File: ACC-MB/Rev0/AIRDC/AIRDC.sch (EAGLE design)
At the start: 4 parts

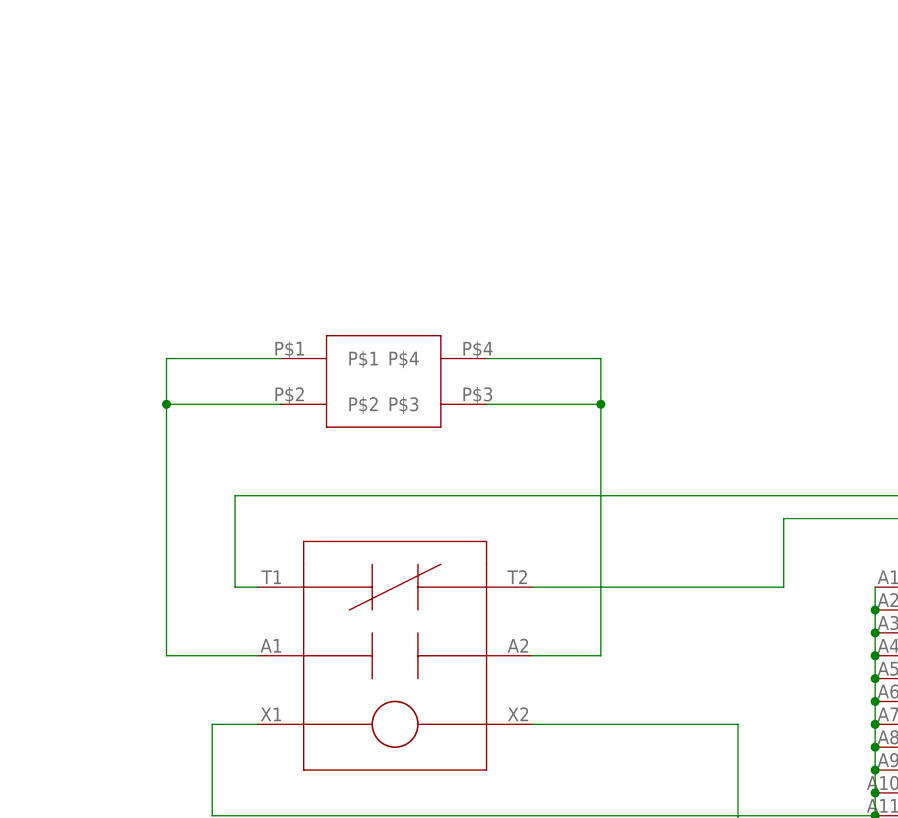
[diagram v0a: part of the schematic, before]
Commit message: update
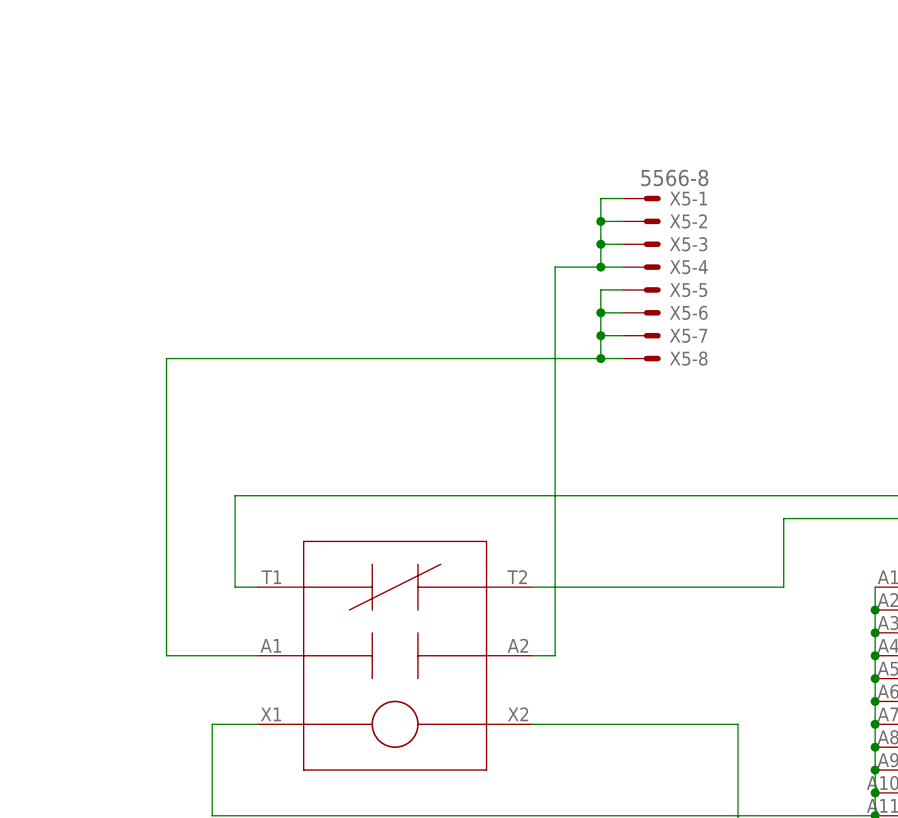
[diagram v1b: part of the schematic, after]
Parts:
- removed U$2: IPBT-102-H1-T-D, ACC-MB-R0:IPBT-102-H1-T-D
- added X5: 5566-8, con-molex:5566-8
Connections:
- removed net N$8: U$1.A2, U$2.P$3, U$2.P$4
- new net N$5: U$1.A1, X5-5.S, X5-6.S, X5-7.S, X5-8.S
- net N$6: now also U$1.A2, X5-1.S, X5-2.S, X5-3.S, X5-4.S; no longer U$1.A1, U$2.P$1, U$2.P$2
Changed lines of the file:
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@@
 <part name="FRAME3" library="ACC-MB-R0" deviceset="A3L-LOC" device=""/>
 <part name="U$1" library="ACC-MB-R0" library_urn="urn:adsk.eagle:library:13324935" deviceset="GV224" device="" package3d_urn="urn:adsk.eagle:package:13209922/2"/>
-<part name="U$2" library="ACC-MB-R0" library_urn="urn:adsk.eagle:library:13324935" deviceset="IPBT-102-H1-T-D" device="" package3d_urn="urn:adsk.eagle:package:13324986/2"/>
 <part name="U$3" library="ACC-MB-R0" library_urn="urn:adsk.eagle:library:13324935" deviceset="PCIE-36-EDGE" device=""/>
 <part name="U$4" library="ACC-MB-R0" library_urn="urn:adsk.eagle:library:13324935" deviceset="PCIE-36-EDGE" device=""/>
+<part name="X5" library="con-molex" library_urn="urn:adsk.eagle:library:165" deviceset="5566-8" device=""/>
 </parts>
 <sheets>
@@
 </instance>
 <instance part="U$1" gate="G$1" x="116.84" y="132.08"/>
-<instance part="U$2" gate="G$1" x="124.46" y="175.26"/>
 <instance part="U$3" gate="G$1" x="185.42" y="157.48"/>
 <instance part="U$4" gate="G$1" x="226.06" y="157.48"/>
+<instance part="X5" gate="-1" x="154.94" y="198.12"/>
+<instance part="X5" gate="-2" x="154.94" y="195.58"/>
+<instance part="X5" gate="-3" x="154.94" y="193.04"/>
+<instance part="X5" gate="-4" x="154.94" y="190.5"/>
+<instance part="X5" gate="-5" x="154.94" y="187.96"/>
+<instance part="X5" gate="-6" x="154.94" y="185.42"/>
+<instance part="X5" gate="-7" x="154.94" y="182.88"/>
+<instance part="X5" gate="-8" x="154.94" y="180.34"/>
 </instances>
 <busses>
@@
 <pinref part="U$3" gate="G$1" pin="A11"/>
 <junction x="180.34" y="129.54"/>
-</segment>
-</net>
-<net name="N$6" class="0">
-<segment>
-<wire x1="111.76" y1="147.32" x2="101.6" y2="147.32" width="0.1524" layer="91"/>
-<wire x1="101.6" y1="147.32" x2="101.6" y2="175.26" width="0.1524" layer="91"/>
-<wire x1="101.6" y1="175.26" x2="114.3" y2="175.26" width="0.1524" layer="91"/>
-<wire x1="114.3" y1="180.34" x2="101.6" y2="180.34" width="0.1524" layer="91"/>
-<wire x1="101.6" y1="180.34" x2="101.6" y2="175.26" width="0.1524" layer="91"/>
-<junction x="101.6" y="175.26"/>
-<pinref part="U$1" gate="G$1" pin="A1"/>
-<pinref part="U$2" gate="G$1" pin="P$1"/>
-<pinref part="U$2" gate="G$1" pin="P$2"/>
-</segment>
-</net>
-<net name="N$8" class="0">
-<segment>
-<wire x1="137.16" y1="175.26" x2="149.86" y2="175.26" width="0.1524" layer="91"/>
-<wire x1="149.86" y1="175.26" x2="149.86" y2="147.32" width="0.1524" layer="91"/>
-<wire x1="149.86" y1="147.32" x2="142.24" y2="147.32" width="0.1524" layer="91"/>
-<wire x1="137.16" y1="180.34" x2="149.86" y2="180.34" width="0.1524" layer="91"/>
-<wire x1="149.86" y1="180.34" x2="149.86" y2="175.26" width="0.1524" layer="91"/>
-<junction x="149.86" y="175.26"/>
-<pinref part="U$1" gate="G$1" pin="A2"/>
-<pinref part="U$2" gate="G$1" pin="P$3"/>
-<pinref part="U$2" gate="G$1" pin="P$4"/>
 </segment>
 </net>
@@
 </segment>
 </net>
+<net name="N$5" class="0">
+<segment>
+<wire x1="111.76" y1="147.32" x2="101.6" y2="147.32" width="0.1524" layer="91"/>
+<pinref part="U$1" gate="G$1" pin="A1"/>
+<wire x1="101.6" y1="147.32" x2="101.6" y2="170.18" width="0.1524" layer="91"/>
+<pinref part="X5" gate="-5" pin="S"/>
+<wire x1="149.86" y1="180.34" x2="149.86" y2="182.88" width="0.1524" layer="91"/>
+<wire x1="149.86" y1="182.88" x2="149.86" y2="185.42" width="0.1524" layer="91"/>
+<wire x1="149.86" y1="185.42" x2="149.86" y2="187.96" width="0.1524" layer="91"/>
+<wire x1="149.86" y1="187.96" x2="152.4" y2="187.96" width="0.1524" layer="91"/>
+<pinref part="X5" gate="-6" pin="S"/>
+<wire x1="152.4" y1="185.42" x2="149.86" y2="185.42" width="0.1524" layer="91"/>
+<junction x="149.86" y="185.42"/>
+<pinref part="X5" gate="-7" pin="S"/>
+<wire x1="152.4" y1="182.88" x2="149.86" y2="182.88" width="0.1524" layer="91"/>
+<junction x="149.86" y="182.88"/>
+<pinref part="X5" gate="-8" pin="S"/>
+<wire x1="152.4" y1="180.34" x2="149.86" y2="180.34" width="0.1524" layer="91"/>
+<wire x1="101.6" y1="170.18" x2="101.6" y2="180.34" width="0.1524" layer="91"/>
+<wire x1="101.6" y1="180.34" x2="149.86" y2="180.34" width="0.1524" layer="91"/>
+<junction x="149.86" y="180.34"/>
+</segment>
+</net>
+<net name="N$6" class="0">
+<segment>
+<pinref part="X5" gate="-3" pin="S"/>
+<pinref part="X5" gate="-1" pin="S"/>
+<wire x1="149.86" y1="198.12" x2="152.4" y2="198.12" width="0.1524" layer="91"/>
+<pinref part="X5" gate="-2" pin="S"/>
+<wire x1="152.4" y1="195.58" x2="149.86" y2="195.58" width="0.1524" layer="91"/>
+<wire x1="149.86" y1="195.58" x2="149.86" y2="198.12" width="0.1524" layer="91"/>
+<junction x="149.86" y="195.58"/>
+<wire x1="149.86" y1="195.58" x2="149.86" y2="193.04" width="0.1524" layer="91"/>
+<wire x1="149.86" y1="193.04" x2="152.4" y2="193.04" width="0.1524" layer="91"/>
+<junction x="149.86" y="193.04"/>
+<pinref part="X5" gate="-4" pin="S"/>
+<wire x1="152.4" y1="190.5" x2="149.86" y2="190.5" width="0.1524" layer="91"/>
+<wire x1="149.86" y1="190.5" x2="149.86" y2="193.04" width="0.1524" layer="91"/>
+<pinref part="U$1" gate="G$1" pin="A2"/>
+<wire x1="142.24" y1="147.32" x2="144.78" y2="147.32" width="0.1524" layer="91"/>
+<wire x1="144.78" y1="147.32" x2="144.78" y2="190.5" width="0.1524" layer="91"/>
+<wire x1="144.78" y1="190.5" x2="149.86" y2="190.5" width="0.1524" layer="91"/>
+<junction x="149.86" y="190.5"/>
+</segment>
+</net>
